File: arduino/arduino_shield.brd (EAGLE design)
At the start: 100 x 80 mm, 14 parts, among them IC3 PCF8574T, IC4 PCF8574T

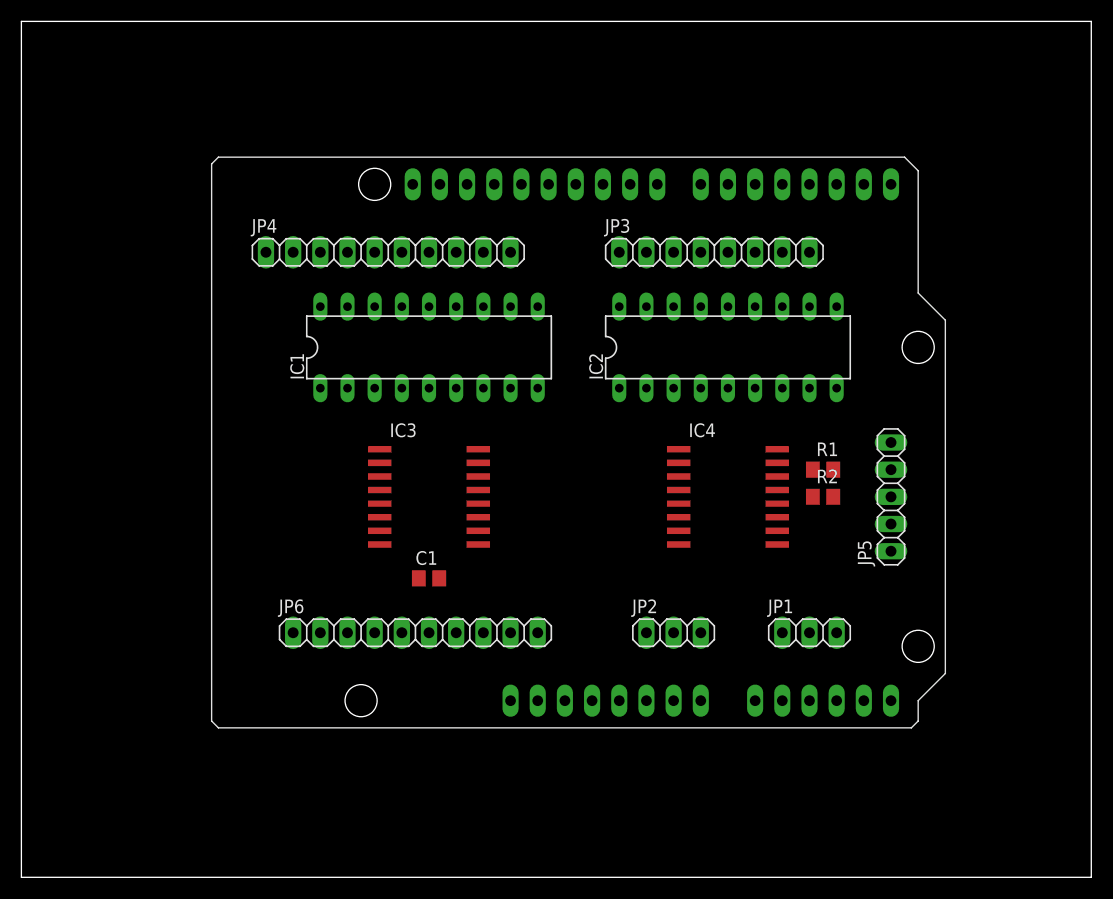
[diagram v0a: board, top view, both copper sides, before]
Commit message: Board erstellt
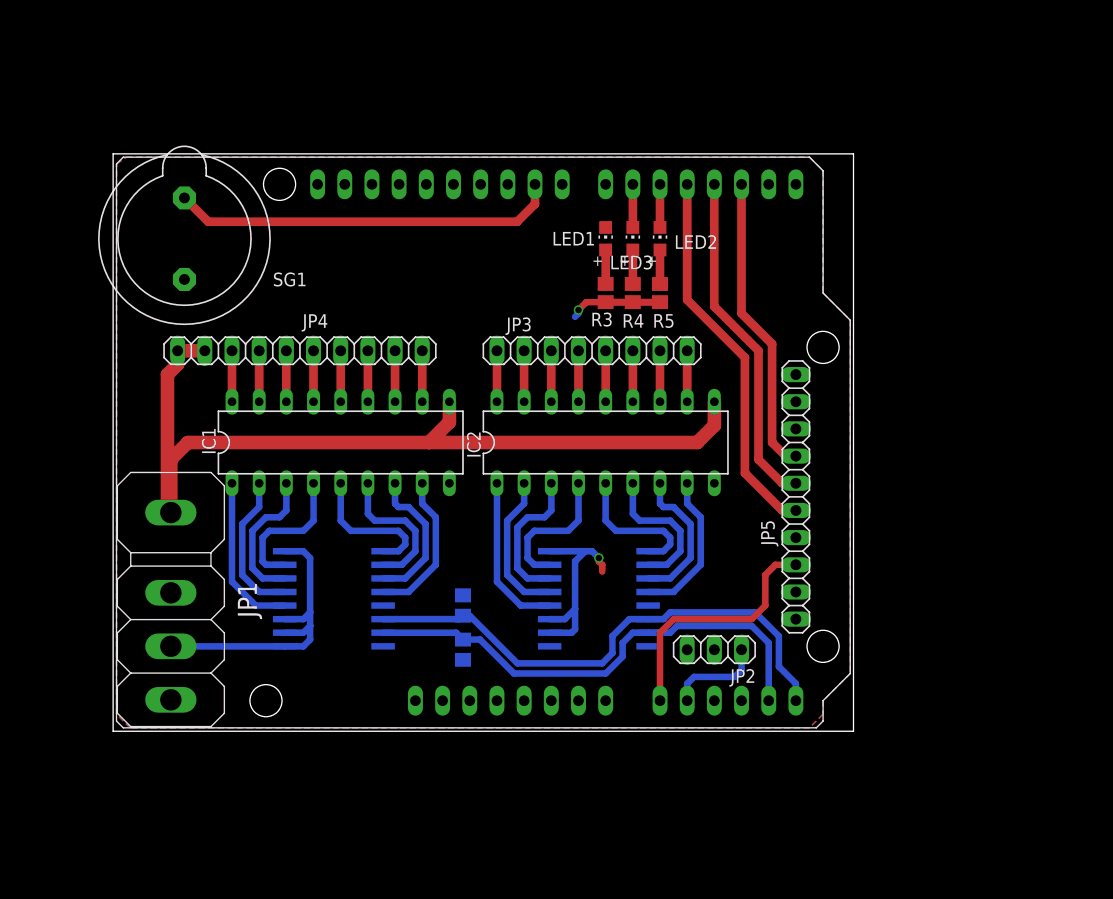
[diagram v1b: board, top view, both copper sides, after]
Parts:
- removed C1: (no value), rcl:C0805
- removed JP6: (no value), pinheader_250:1X10
- added LED1, LED2, LED3: (no value), adafruit:CHIP-LED0805
- added R3, R4, R5: (no value), resistor:R0805
- added SG1: F/HGP, buzzer:F/HGP
- added U$1: (no value), frames:A4L-LOC
- JP1: value (none) -> POWERCON; device pinheader_250:1X03 -> PowerCon:AYAB_POW
- JP5: device pinheader_250:1X05 -> pinheader_250:1X10
- moved JP1 59.7 mm to (14.0, 21.6), turned to 90 degrees
- moved R1 37.6 mm to (41.3, 21.3), flipped to the bottom, turned to 270 degrees
- moved R2 35.2 mm to (41.3, 25.4), flipped to the bottom, turned to 90 degrees
- moved IC4 15.4 mm to (54.0, 26.0), flipped to the bottom, turned to 90 degrees
- moved JP3 14.7 mm to (53.3, 49.2)
- moved IC2 14.5 mm to (54.6, 40.6)
- moved IC3 13.0 mm to (29.2, 26.0), flipped to the bottom, turned to 90 degrees
- moved JP4 12.4 mm to (26.0, 49.2)
- moved IC1 12.1 mm to (29.8, 40.6)
- moved ARD1 8.89 mm to (8.89, 14.0)
- moved JP5 8.89 mm to (72.4, 35.6), turned to 270 degrees
- moved JP2 4.13 mm to (64.8, 21.3), turned to 180 degrees
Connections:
- net EOL_R renamed EOL0L
- removed net 5V: ARD1.5V
- removed net AREF: ARD1.AREF
- removed net EOL_L: ARD1.AIN0, JP1.1
- removed net GND1: ARD1.GND@1, ARD1.GND@2, ARD1.GND@3, C1.2, IC1.9, IC2.9, IC3.1, IC3.2, IC3.3, IC3.8, IC4.2, IC4.3, IC4.8, JP1.2, JP2.2, JP5.4, JP6.7
- removed net INT0: ARD1.2
- removed net INT1: ARD1.3
- removed net V+: IC1.10, IC2.10, JP4.1, JP4.2, JP6.10
- new net +15V: IC1.10, IC2.10, JP1.P$1, JP4.1, JP4.2
- new net +5V/1: JP1.P$4
- new net ENC0PINA: ARD1.2, JP5.4
- new net ENC0PINB: ARD1.3, JP5.5
- new net ENC0PINC: ARD1.4, JP5.6
- new net EOL0R: ARD1.AIN0, JP5.8
- new net GND: ARD1.GND@1, ARD1.GND@2, ARD1.GND@3, IC1.9, IC2.9, IC3.1, IC3.2, IC3.3, IC3.8, IC4.2, IC4.3, IC4.8, JP1.P$2, JP1.P$3, JP2.2, JP5.10, JP5.2, JP5.7, JP5.9, LED1.C
- new net N$33: LED1.A, R3.1
- new net N$34: ARD1.9, SG1.1
- new net N$35: ARD1.6, LED3.C
- new net N$36: ARD1.5, LED2.C
- new net N$37: LED3.A, R4.2
- new net N$38: LED2.A, R5.2
- net +5V: now also ARD1.5V, ARD1.AREF, IC4.1, JP5.1, R3.2, R4.1, R5.1, SG1.2; no longer C1.1, JP1.3, JP5.5, JP6.3
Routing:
- net +15V: track 0.00 -> 82.1 mm
- net SCL: track 0.00 -> 49.5 mm
- net GND: track 0.00 -> 48.2 mm, vias 0 -> 1
- net SDA: track 0.00 -> 46.3 mm
- net N$34: track 0.00 -> 36.2 mm
- net ENC0PINC: track 0.00 -> 35.4 mm
- net ENC0PINB: track 0.00 -> 31.8 mm
- net ENC0PINA: track 0.00 -> 28.1 mm
- net EOL0R: track 0.00 -> 23.4 mm
- net N$2: track 0.00 -> 15.1 mm
- net N$1: track 0.00 -> 15.1 mm
- net N$16: track 0.00 -> 14.1 mm
- net N$9: track 0.00 -> 14.1 mm
- net N$3: track 0.00 -> 13.9 mm
- net N$10: track 0.00 -> 13.9 mm
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- added copper zone on layer 16, net +5V
- added copper zone on layer 1, net GND
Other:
- board size 100 x 80 mm -> 69.2 x 54 mm
